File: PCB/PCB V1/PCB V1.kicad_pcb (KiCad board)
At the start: 2 copper layers, 100 x 100 mm, 48 parts, among them J1 Screw_Terminal_01x03, J2 Screw_Terminal_01x03, J3 USB_B, J4 Conn_01x02_Pin, K1 Relay_SPDT, K2 Relay_SPDT, Q1 S8050, Q2 S8050, Q3 S8050, SW1 On/Off, SW2 SW_Push, SW3 SW_Push, U1 LM317_TO-220

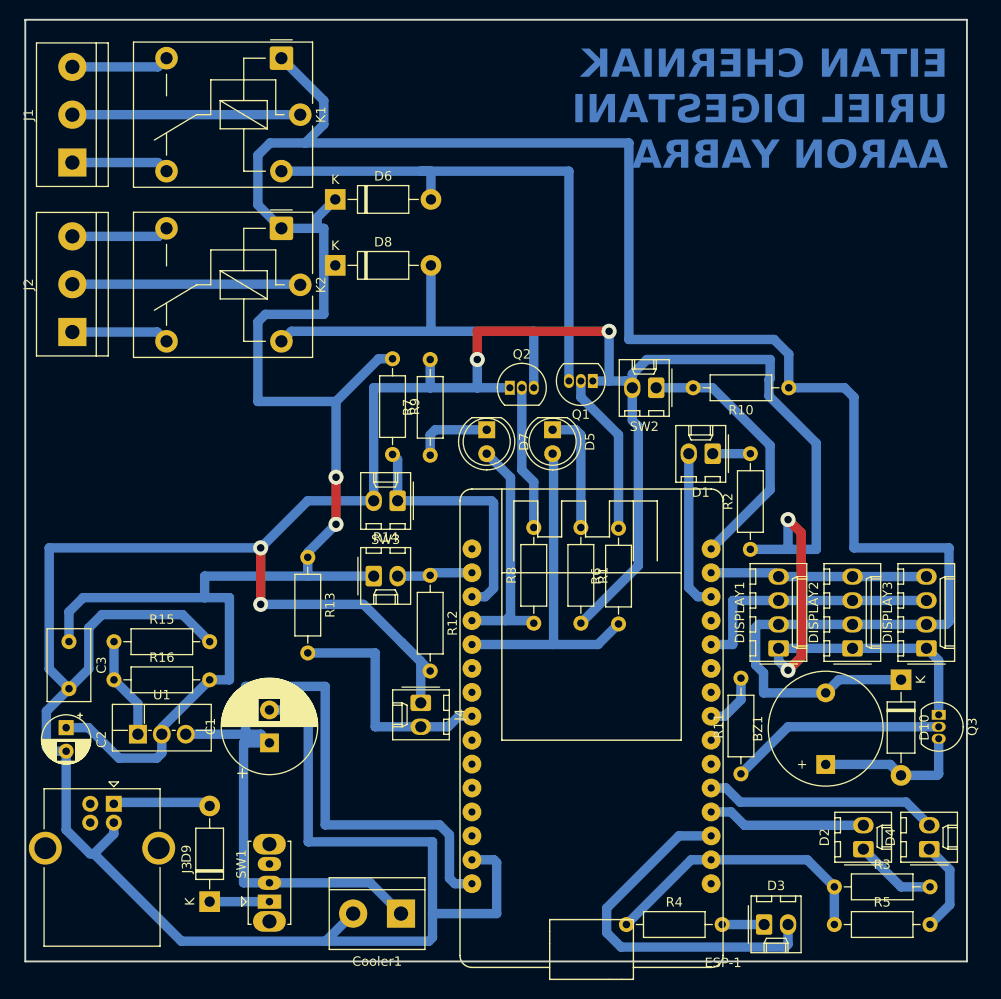
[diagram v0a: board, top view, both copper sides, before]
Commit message: Update PCB V1.kicad_pcb
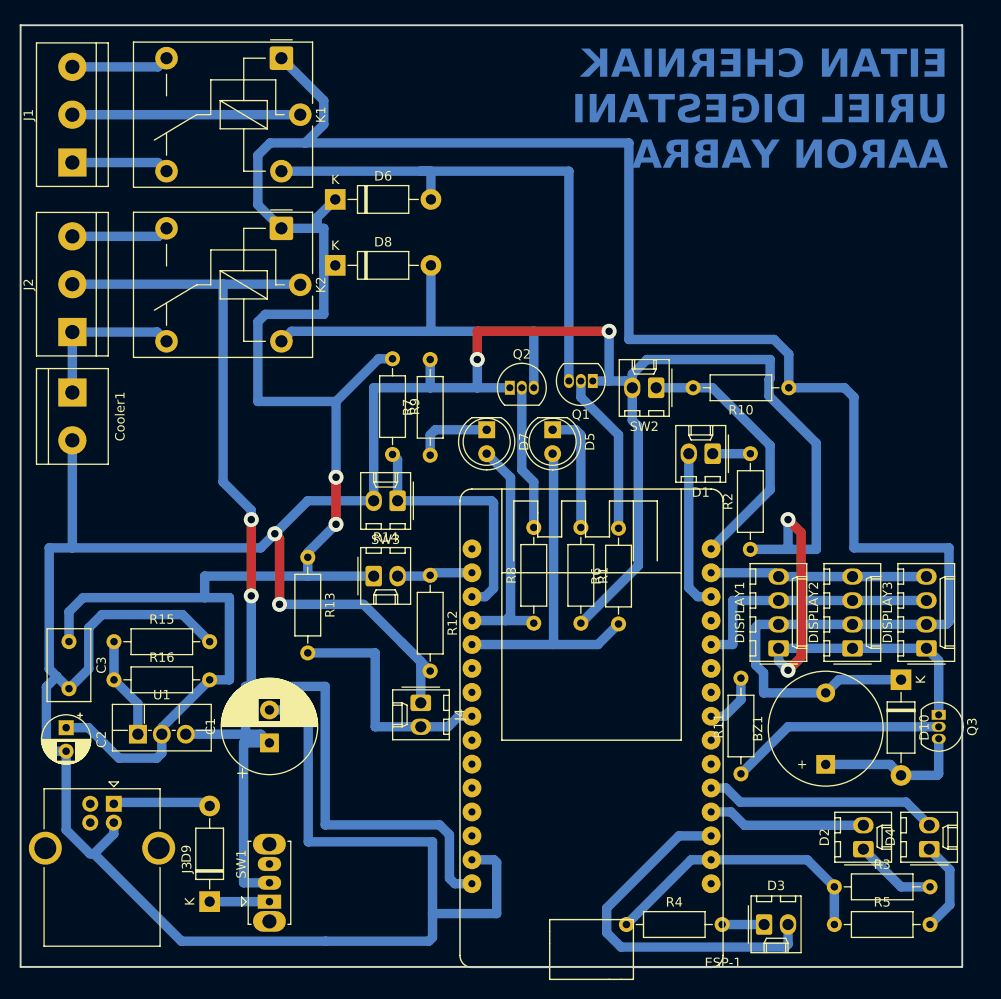
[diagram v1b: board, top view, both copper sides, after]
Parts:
- moved Cooler1 65.4 mm to (54.0, 61.5), turned to -90 degrees
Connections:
- Cooler1 pad 1: +5V -> NO
- J2 pad 1: Net-(J2-Pin_1) -> NO
- J2 pad 2: Net-(J2-Pin_2) -> +5V
- K2 pad 11: Net-(J2-Pin_2) -> +5V
- K2 pad 12: Net-(J2-Pin_1) -> NO
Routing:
- net +5V: track 94.1 -> 146.9 mm, vias 0 -> 2
- net Net-(J2-Pin_2): track 24.2 -> 0.00 mm
- net NO: track 0.00 -> 16.8 mm
- net Net-(J2-Pin_1): track 10.4 -> 0.00 mm
- net GND: track 444.8 -> 452.3 mm
